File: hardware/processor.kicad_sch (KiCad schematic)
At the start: 25 parts, among them J10 FAULT, J11 PWR, J12 GPS, J13 HIGH, J14 LOW, J15 LOCK, J16 Program/Run, J17 ICSP, J7 LCD, J8 SPARE 1, J9 SPARE 2, Q1 2N3904, SW2 SW_DIP_x08, U7 MCP23017_SO, U8 MCP23017_SO, U9 PIC18F27Q43

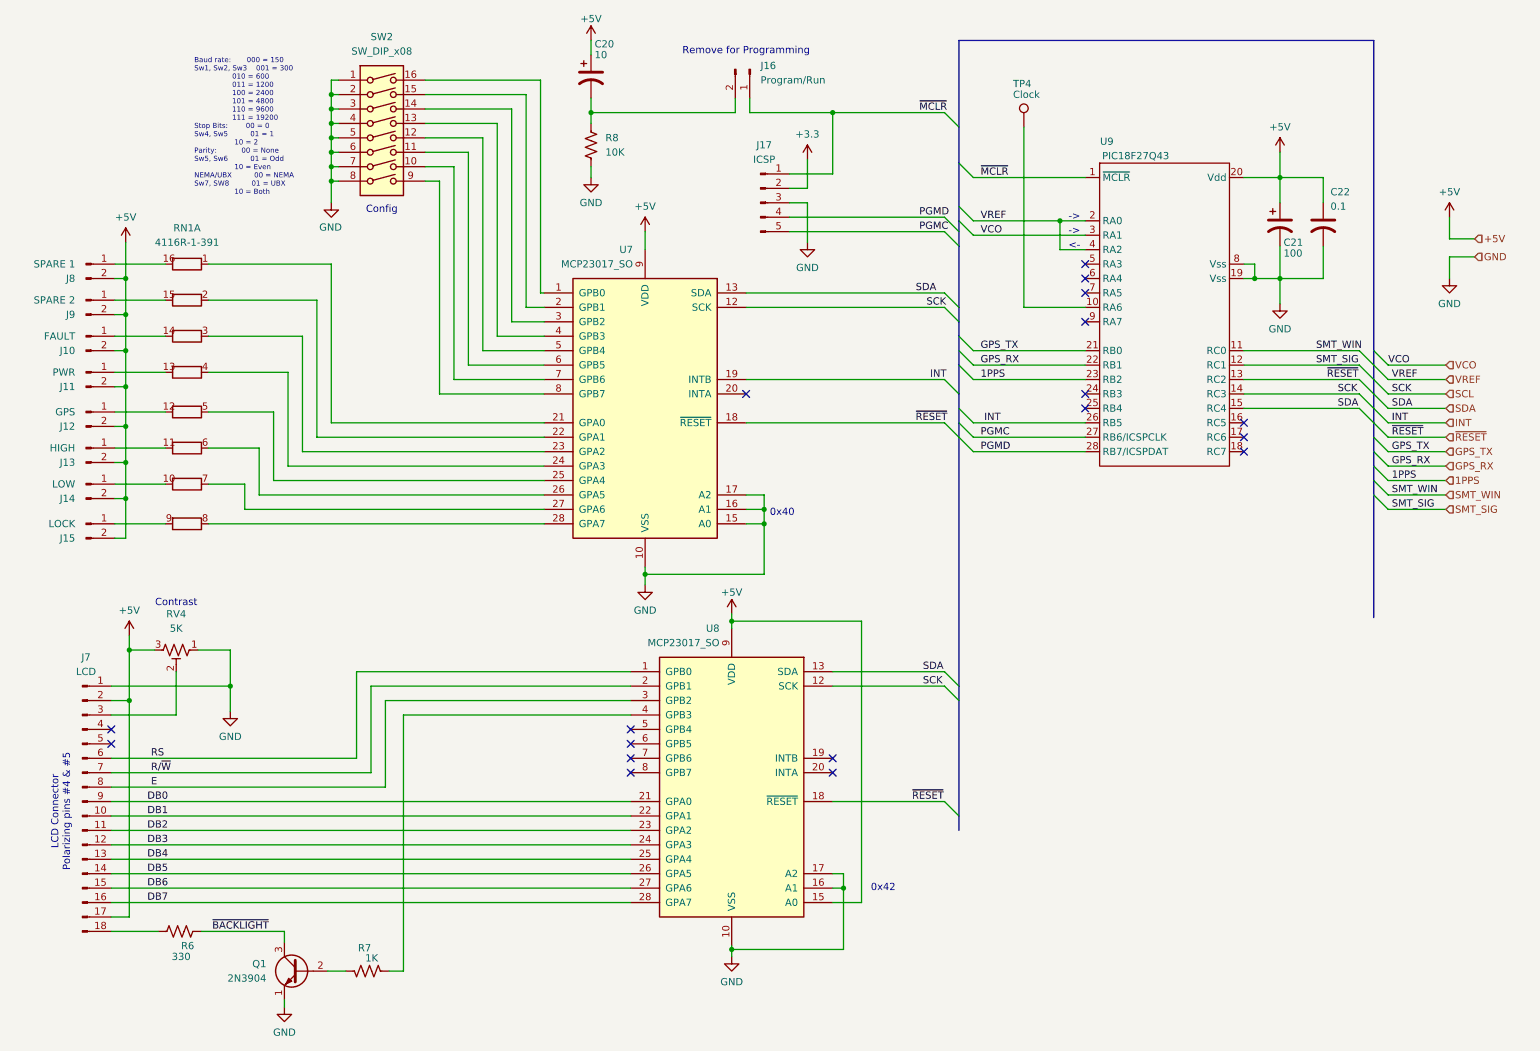
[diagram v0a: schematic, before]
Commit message: Revised hardware design
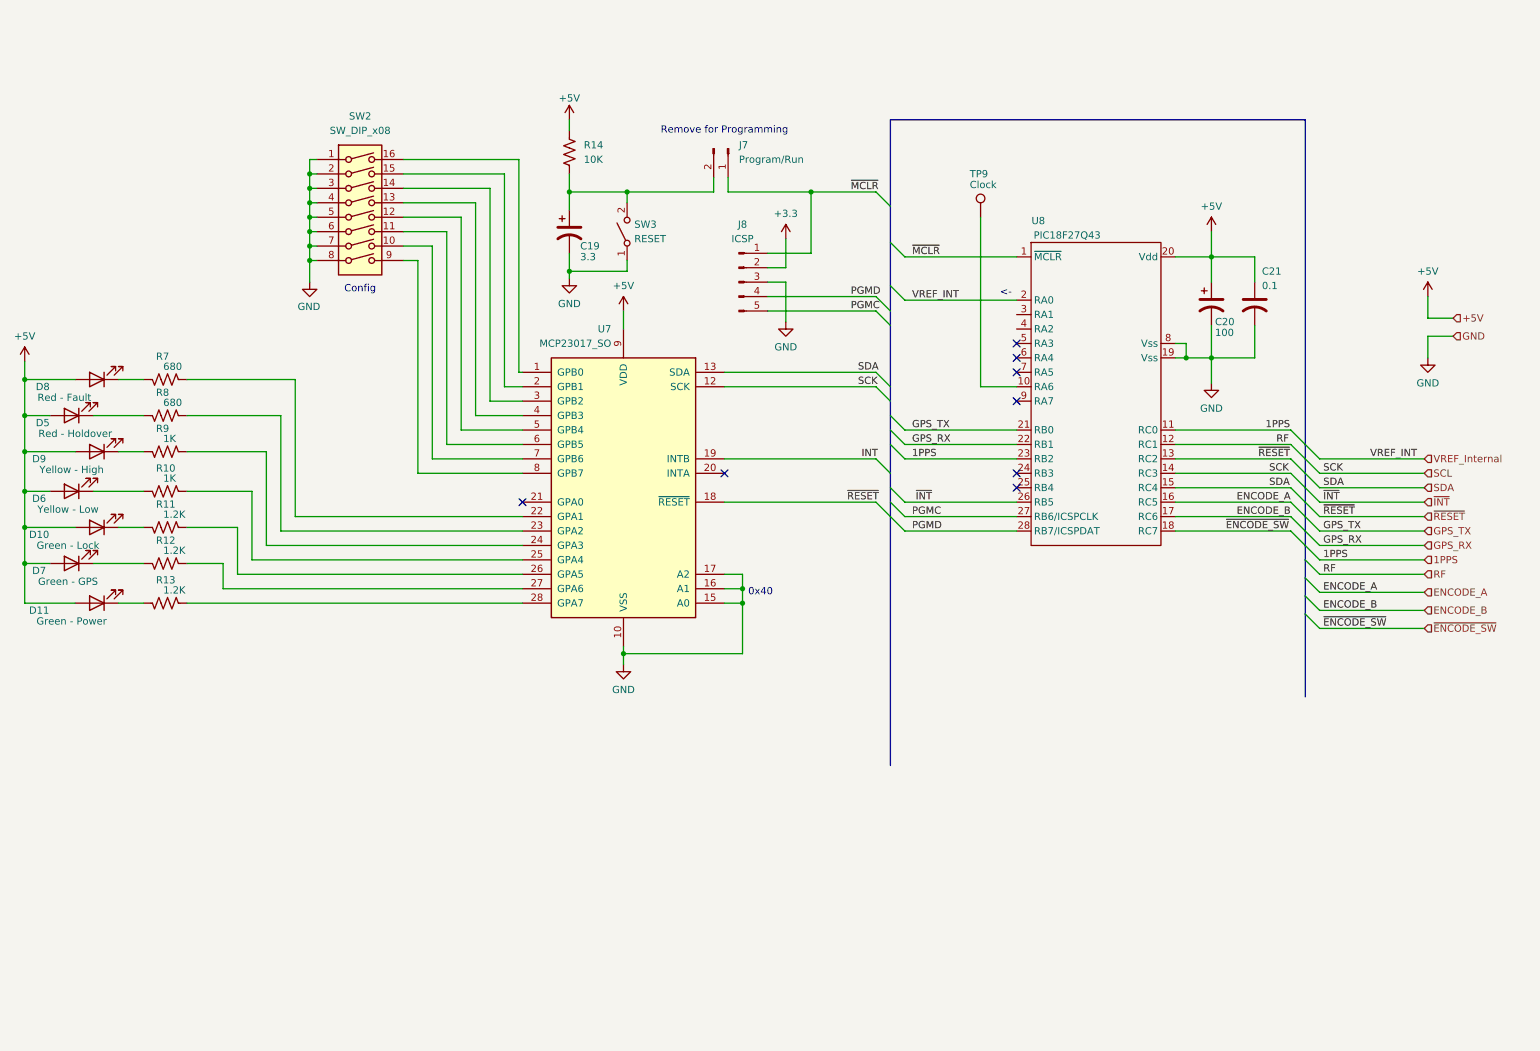
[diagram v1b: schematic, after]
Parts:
- removed J10: FAULT, Connector_PinHeader_2.54mm:PinHeader_1x02_P2.54mm_Vertical, symbol Connector:Conn_01x02_Pin
- removed J11: PWR, Connector_PinHeader_2.54mm:PinHeader_1x02_P2.54mm_Vertical, symbol Connector:Conn_01x02_Pin
- removed J12: GPS, Connector_PinHeader_2.54mm:PinHeader_1x02_P2.54mm_Vertical, symbol Connector:Conn_01x02_Pin
- removed J13: HIGH, Connector_PinHeader_2.54mm:PinHeader_1x02_P2.54mm_Vertical, symbol Connector:Conn_01x02_Pin
- removed J14: LOW, Connector_PinHeader_2.54mm:PinHeader_1x02_P2.54mm_Vertical, symbol Connector:Conn_01x02_Pin
- removed J15: LOCK, Connector_PinHeader_2.54mm:PinHeader_1x02_P2.54mm_Vertical, symbol Connector:Conn_01x02_Pin
- removed J7: LCD, Connector_PinHeader_2.54mm:PinHeader_1x18_P2.54mm_Vertical, symbol Connector:Conn_01x18_Pin
- removed J8: SPARE 1, Connector_PinHeader_2.54mm:PinHeader_1x02_P2.54mm_Vertical, symbol Connector:Conn_01x02_Pin
- removed J9: SPARE 2, Connector_PinHeader_2.54mm:PinHeader_1x02_P2.54mm_Vertical, symbol Connector:Conn_01x02_Pin
- removed Q1: 2N3904, Package_TO_SOT_THT:TO-92_Inline, symbol Transistor_BJT:2N3904
- removed R6: 330, Resistor_SMD:R_0805_2012Metric_Pad1.20x1.40mm_HandSolder, symbol Device:R_US
- removed RN1: 4116R-1-391, Package_DIP:DIP-16_W7.62mm_LongPads, symbol Device:R_Pack08_Split
- removed RV4: 5K, Potentiometer_THT:Potentiometer_Bourns_3296W_Vertical, symbol Device:R_Potentiometer_Trim_US
- removed U8: MCP23017_SO, Package_SO:SOIC-28W_7.5x17.9mm_P1.27mm, symbol Interface_Expansion:MCP23017_SO
- added D10: Green - Lock, symbol Device:LED
- added D11: Green - Power, symbol Device:LED
- added D5: Red - Holdover, symbol Device:LED
- added D6: Yellow - Low, symbol Device:LED
- added D7: Green - GPS, symbol Device:LED
- added D8: Red - Fault, symbol Device:LED
- added D9: Yellow - High, symbol Device:LED
- added R10, R9: 1K, Resistor_SMD:R_0805_2012Metric_Pad1.20x1.40mm_HandSolder, symbol Device:R_US
- added R11, R12, R13: 1.2K, Resistor_SMD:R_0805_2012Metric_Pad1.20x1.40mm_HandSolder, symbol Device:R_US
- added R8: 680, Resistor_SMD:R_0805_2012Metric_Pad1.20x1.40mm_HandSolder, symbol Device:R_US
- added SW3: RESET, symbol Switch:SW_SPST
- C19: renamed from C20; value 10 -> 3.3
- R7: value 1K -> 680
- renumbered C21 to C20, C22 to C21, J16 to J7, J17 to J8, R8 to R14, TP4 to TP9, U9 to U8
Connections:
- net SMT_WIN is gone; now on net 1PPS: U8.11 (RC0)
- net +5V: now also R14.1, D10.2 (A), D11.2 (A), D5.2 (A), D6.2 (A), D7.2 (A), D8.2 (A), D9.2 (A); no longer C19.1
- net GND: now also C19.2, SW3.1 (A); no longer R14.2
- net INT: no longer U8.26 (RB5)
- net at U7.23 (GPA2): now also R8.1
- net at U7.25 (GPA4): now also R10.1
- net at U7.24 (GPA3): now also R9.1
- net at R7.2: now also D8.1 (K)
- net at U7.22 (GPA1): now also R7.1
- net at U7.26 (GPA5): now also R11.1
- net at U7.27 (GPA6): now also R12.1
- net at U7.28 (GPA7): now also R13.1
- net ENCODE_A: now reaches U8.16 (RC5)
- net ENCODE_B: now reaches U8.17 (RC6)
- net ~{ENCODE_SW}: now reaches U8.18 (RC7)
- net SMT_SIG renamed RF
- net VCO: no longer names the net of U8.3 (RA1)
- net VREF: no longer names the net of U8.4 (RA2)
- net VREF: no longer U8.2 (RA0)
- new net: D11.1 (K), R13.2
- new net: C19.1, J7.2 (Pin_2), R14.2, SW3.2 (B)
- new net: D7.1 (K), R12.2
- new net: D5.1 (K), R8.2
- new net: D10.1 (K), R11.2
- new net: D9.1 (K), R9.2
- new net: D6.1 (K), R10.2
- new net VREF_Internal: U8.2 (RA0)
- new net ~{INT}: U8.26 (RB5)
- no-connect marks 18 -> 8
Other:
- note removed: "->"
- note removed: "0x42"
- note removed: "Baud rate: 000 = 150 Sw1, Sw2, Sw3 001 = 300 010 = 600 011 = 1200 100 = 2400 101 = 4800 110 = 9600 111 = 19200 Stop Bits: 00 = 0 Sw4, Sw5 01 = 1 10 = 2 Parity: 00 = None Sw5, Sw6 01 = Odd 10 = Even NEMA/UBX 00 = NEMA Sw7, SW8 01 = UBX 10 = Both"
- note removed: "Contrast"
- note removed: "LCD Connector Polarizing pins #4 & #5"
- moved on the sheet: C19, C20, C21, J7, J8, R14, SW2, TP9, U7, U8
